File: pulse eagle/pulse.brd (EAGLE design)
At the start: 21 x 31.1 mm, 25 parts, among them IC1 LM358D, J1 ISP Touch, T1 BC846, Y1 8MHz

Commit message: Rev. A of the board.
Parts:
- C1, C3: value .1uf -> 1uf
- C12: value .1uf -> .1uF
- C2, C4: value 15pF -> .1uF
- R2: value 220 -> 39k
- R3, R5: value 220 -> 68k
- R4: value 220 -> 8.2k
- R6: value 220 -> 1k
- R7: value 220 -> 470k
- R8: value 220 -> 1.8k
- T1: value BC846 -> MMBT3904
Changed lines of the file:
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@@
 <attribute name="VALUE" x="7.9756" y="20.1168" size="2.0828" layer="27" ratio="10" rot="SR0"/>
 </element>
-<element name="C12" library="adafruit" package="C0805" value=".1uf" x="18.415" y="11.43" smashed="yes">
+<element name="C12" library="adafruit" package="C0805" value=".1uF" x="18.415" y="11.43" smashed="yes">
 <attribute name="NAME" x="19.14525" y="12.79525" size="0.508" layer="25" rot="R180"/>
 </element>
@@
 <attribute name="NAME" x="14.986" y="19.65325" size="0.4064" layer="25" font="vector"/>
 </element>
-<element name="R2" library="SparkFun-Resistors" package="0603-RES" value="220" x="4.445" y="22.86" smashed="yes" rot="R180">
+<element name="R2" library="SparkFun-Resistors" package="0603-RES" value="39k" x="4.445" y="22.86" smashed="yes" rot="R180">
 <attribute name="PROD_ID" value="RES-07866" x="-26.035" y="64.77" size="1.778" layer="27" rot="R180" display="off"/>
 <attribute name="NAME" x="6.00075" y="23.27275" size="0.4064" layer="25" font="vector" rot="R270"/>
 </element>
-<element name="R3" library="SparkFun-Resistors" package="0603-RES" value="220" x="3.175" y="27.94" smashed="yes" rot="R180">
+<element name="R3" library="SparkFun-Resistors" package="0603-RES" value="68k" x="3.175" y="27.94" smashed="yes" rot="R180">
 <attribute name="PROD_ID" value="RES-07866" x="-31.115" y="69.85" size="1.778" layer="27" rot="R180" display="off"/>
 <attribute name="NAME" x="4.73075" y="28.35275" size="0.4064" layer="25" font="vector" rot="R270"/>
 </element>
-<element name="R4" library="SparkFun-Resistors" package="0603-RES" value="220" x="6.985" y="29.21" smashed="yes">
+<element name="R4" library="SparkFun-Resistors" package="0603-RES" value="8.2k" x="6.985" y="29.21" smashed="yes">
 <attribute name="PROD_ID" value="RES-07866" x="45.085" y="-12.7" size="1.778" layer="27" display="off"/>
 <attribute name="NAME" x="6.731" y="29.81325" size="0.4064" layer="25" font="vector"/>
 </element>
-<element name="R5" library="SparkFun-Resistors" package="0603-RES" value="220" x="18.415" y="29.21" smashed="yes" rot="R180">
+<element name="R5" library="SparkFun-Resistors" package="0603-RES" value="68k" x="18.415" y="29.21" smashed="yes" rot="R180">
 <attribute name="PROD_ID" value="RES-07866" x="-23.495" y="71.12" size="1.778" layer="27" rot="R180" display="off"/>
 <attribute name="NAME" x="18.82775" y="30.19425" size="0.4064" layer="25" font="vector" rot="R180"/>
 </element>
-<element name="R6" library="SparkFun-Resistors" package="0603-RES" value="220" x="18.415" y="26.67" smashed="yes" rot="R180">
+<element name="R6" library="SparkFun-Resistors" package="0603-RES" value="1k" x="18.415" y="26.67" smashed="yes" rot="R180">
 <attribute name="PROD_ID" value="RES-07866" x="-27.305" y="68.58" size="1.778" layer="27" rot="R180" display="off"/>
 <attribute name="NAME" x="16.47825" y="27.08275" size="0.4064" layer="25" font="vector" rot="R270"/>
 </element>
-<element name="R7" library="SparkFun-Resistors" package="0603-RES" value="220" x="18.415" y="22.86" smashed="yes" rot="R180">
+<element name="R7" library="SparkFun-Resistors" package="0603-RES" value="470k" x="18.415" y="22.86" smashed="yes" rot="R180">
 <attribute name="PROD_ID" value="RES-07866" x="3.175" y="68.58" size="1.778" layer="27" rot="R180" display="off"/>
 <attribute name="NAME" x="16.47825" y="23.27275" size="0.4064" layer="25" font="vector" rot="R270"/>
 </element>
-<element name="R8" library="SparkFun-Resistors" package="0603-RES" value="220" x="18.415" y="20.32" smashed="yes">
+<element name="R8" library="SparkFun-Resistors" package="0603-RES" value="1.8k" x="18.415" y="20.32" smashed="yes">
 <attribute name="PROD_ID" value="RES-07866" x="37.465" y="-25.4" size="1.778" layer="27" display="off"/>
 <attribute name="NAME" x="18.82775" y="21.30425" size="0.4064" layer="25" font="vector" rot="R180"/>
 </element>
-<element name="C1" library="adafruit" package="C0805" value=".1uf" x="3.175" y="25.4" smashed="yes" rot="R180">
+<element name="C1" library="adafruit" package="C0805" value="1uf" x="3.175" y="25.4" smashed="yes" rot="R180">
 <attribute name="NAME" x="4.826" y="25.9715" size="0.508" layer="25" rot="R270"/>
 </element>
-<element name="C3" library="adafruit" package="C0805" value=".1uf" x="14.605" y="29.21" smashed="yes">
+<element name="C3" library="adafruit" package="C0805" value="1uf" x="14.605" y="29.21" smashed="yes">
 <attribute name="NAME" x="14.19225" y="30.226" size="0.508" layer="25"/>
 </element>
-<element name="C2" library="SparkFun-Passives" package="0805" value="15pF" x="10.795" y="29.21" smashed="yes">
+<element name="C2" library="SparkFun-Passives" package="0805" value=".1uF" x="10.795" y="29.21" smashed="yes">
 <attribute name="NAME" x="10.50925" y="30.0355" size="0.4064" layer="25"/>
 </element>
-<element name="C4" library="SparkFun-Passives" package="0805" value="15pF" x="18.415" y="24.765" smashed="yes">
+<element name="C4" library="SparkFun-Passives" package="0805" value=".1uF" x="18.415" y="24.765" smashed="yes">
 <attribute name="NAME" x="16.9545" y="24.47925" size="0.4064" layer="25" rot="R90"/>
 </element>
-<element name="T1" library="transistor" package="SOT23" value="BC846" x="18.415" y="15.24" smashed="yes" rot="R180">
+<element name="T1" library="transistor" package="SOT23" value="MMBT3904" x="18.415" y="15.24" smashed="yes" rot="R180">
 <attribute name="NAME" x="17.78" y="14.44625" size="0.508" layer="25" rot="R180"/>
 </element>

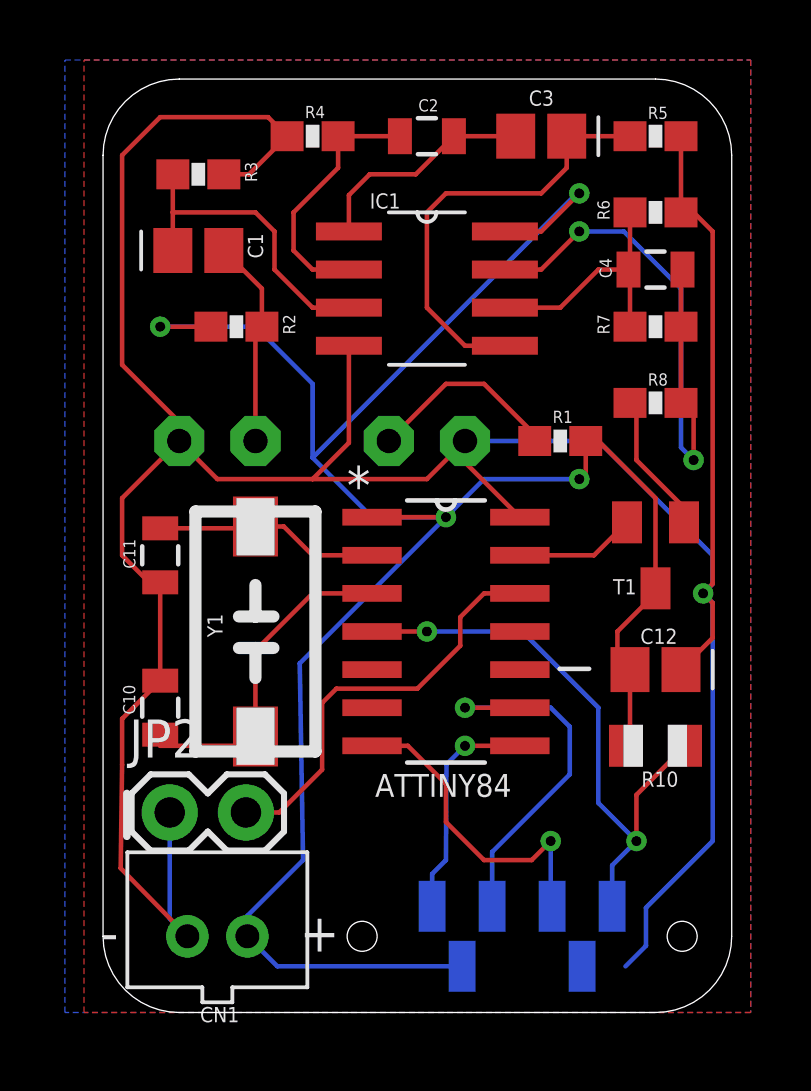
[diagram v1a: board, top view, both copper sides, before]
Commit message: Moving pins around.
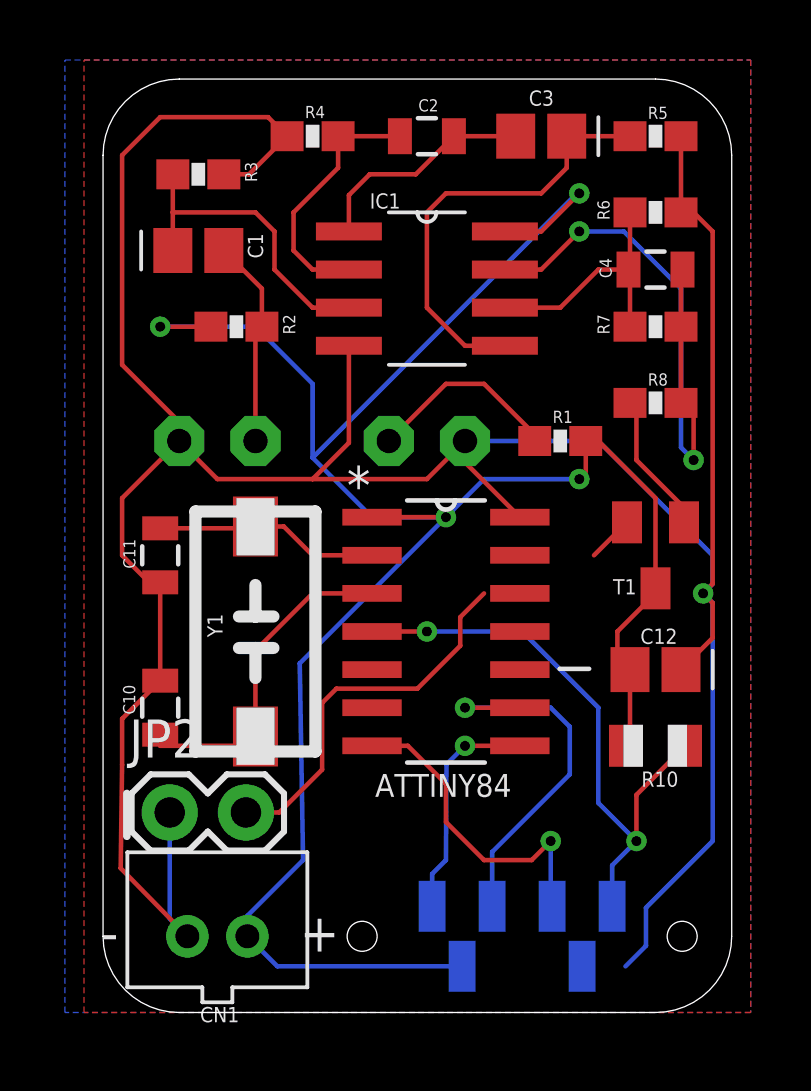
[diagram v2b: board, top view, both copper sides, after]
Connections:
- net A0: now also ATTINY84.12; no longer ATTINY84.13
- net SERIAL: now also ATTINY84.11; no longer ATTINY84.12
- net VCC: now also ATTINY84.13
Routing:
- net A0: track 4.03 -> 1.56 mm
- net SERIAL: track 14.0 -> 12.8 mm
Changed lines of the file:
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@@
 <layer number="112" name="tSilk" color="7" fill="1" visible="yes" active="yes"/>
 <layer number="116" name="Patch_BOT" color="9" fill="4" visible="yes" active="yes"/>
+<layer number="118" name="Rect_Pads" color="7" fill="1" visible="no" active="no"/>
 <layer number="121" name="_tsilk" color="7" fill="1" visible="yes" active="yes"/>
 <layer number="122" name="_bsilk" color="7" fill="1" visible="yes" active="yes"/>
@@
 <wire x1="15.875" y1="27.305" x2="15.7988" y2="27.305" width="0.1524" layer="16"/>
 <wire x1="15.7988" y1="27.305" x2="6.985" y2="18.4912" width="0.1524" layer="16"/>
+<contactref element="ATTINY84" pad="13"/>
+<wire x1="11.43" y1="16.51" x2="13.8938" y2="15.24" width="0" layer="19" extent="1-16"/>
 </signal>
 <signal name="RESET">
@@
 </signal>
 <signal name="A0">
-<contactref element="ATTINY84" pad="13"/>
 <contactref element="T1" pad="2"/>
-<wire x1="13.8938" y1="15.24" x2="16.365" y2="15.24" width="0.1524" layer="1"/>
 <wire x1="16.365" y1="15.24" x2="17.465" y2="16.34" width="0.1524" layer="1"/>
+<contactref element="ATTINY84" pad="12"/>
+<wire x1="13.8938" y1="13.97" x2="16.365" y2="15.24" width="0" layer="19" extent="1-1"/>
 </signal>
 <signal name="SERIAL">
-<contactref element="ATTINY84" pad="12"/>
 <contactref element="JP2" pad="2"/>
 <wire x1="4.7625" y1="6.6675" x2="5.87375" y2="6.6675" width="0.1524" layer="1"/>
@@
 <wire x1="11.90625" y1="12.22375" x2="11.90625" y2="13.17625" width="0.1524" layer="1"/>
 <wire x1="11.90625" y1="13.17625" x2="12.7" y2="13.97" width="0.1524" layer="1"/>
-<wire x1="12.7" y1="13.97" x2="13.8938" y2="13.97" width="0.1524" layer="1"/>
+<contactref element="ATTINY84" pad="11"/>
+<wire x1="12.7" y1="13.97" x2="13.8938" y2="12.7" width="0" layer="19" extent="1-1"/>
 </signal>
 </signals>
